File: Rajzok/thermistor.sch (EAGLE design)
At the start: 17 parts, among them Q1 TP0602N2, Q2 TP0602N2, Q3 SUP75N06-08, Q4 SUP75N06-08

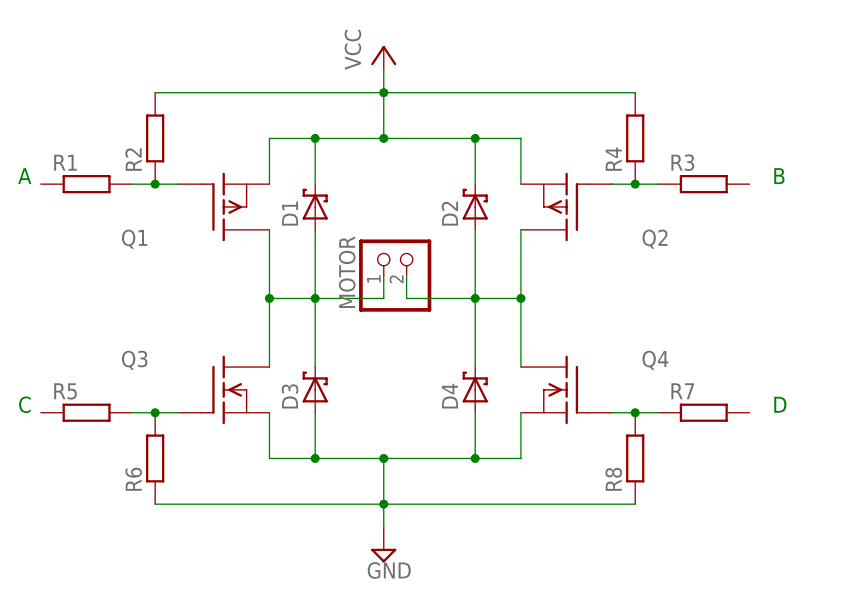
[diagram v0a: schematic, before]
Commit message: Rajzok 2017
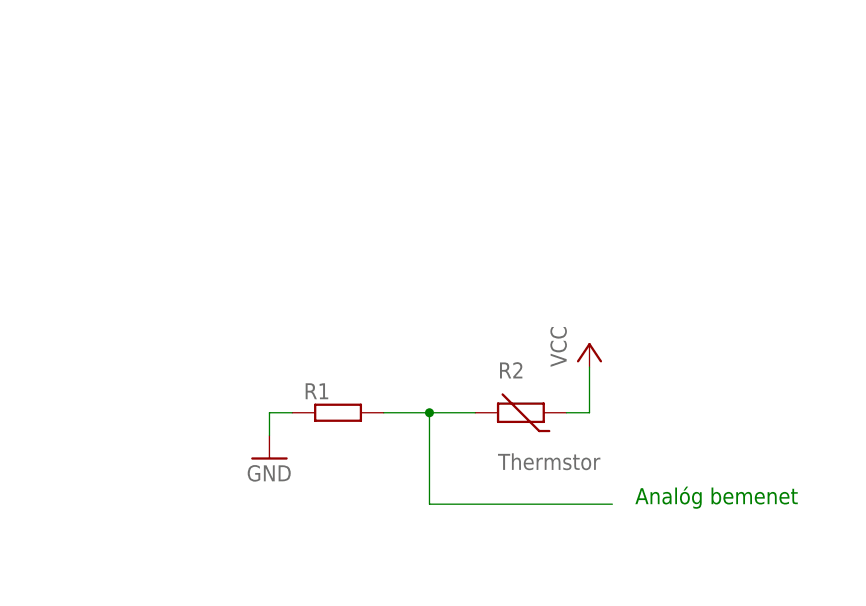
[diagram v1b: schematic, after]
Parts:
- removed D1, D2, D3, D4: 1N6267A, diode:1N6267A
- removed MOTOR: (no value), pinhead:PINHD-1X2
- removed Q1, Q2: TP0602N2, transistor-fet:TP0602N2
- removed Q3, Q4: SUP75N06-08, transistor-fet:SUP75N06-08
- removed R3, R4, R5, R6, R7, R8: (no value), rcl:R-EU_0204/7
- R1: device rcl:R-EU_0204/7 -> resistor:R-EU_0204/7
- R2: value (none) -> Thermstor; device rcl:R-EU_0204/7 -> varistor:THERMISTOR-5
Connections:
- removed net N$2: D2.A, D4.C, MOTOR.2, Q2.D, Q4.D
- removed net N$3: Q2.G, R3.1, R4.1
- removed net N$4: Q3.G, R5.2, R6.2
- removed net N$5: Q4.G, R7.1, R8.2
- removed net N$9: D1.A, D3.C, MOTOR.1, Q1.D, Q3.D
- net GND: now also R1.1; no longer D3.A, D4.A, Q3.S, Q4.S, R6.1, R8.1
- net N$1: now also R2.2; no longer Q1.G, R2.1
- net VCC: now also R2.1; no longer D1.C, D2.C, Q1.S, Q2.S, R2.2, R4.2
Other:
- note added: "Analóg bemenet"
- note removed: "A"
- note removed: "B"
- note removed: "C"
- note removed: "D"
- moved on the sheet: R1
